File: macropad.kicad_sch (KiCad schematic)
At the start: 6 parts, among them J1 OLED_128x32, SW1 SW_Push, SW2 SW_Push, SW3 SW_Push, SW4 RotaryEncoder_Switch, U1 MOUDLE-SEEEDUINO-XIAO

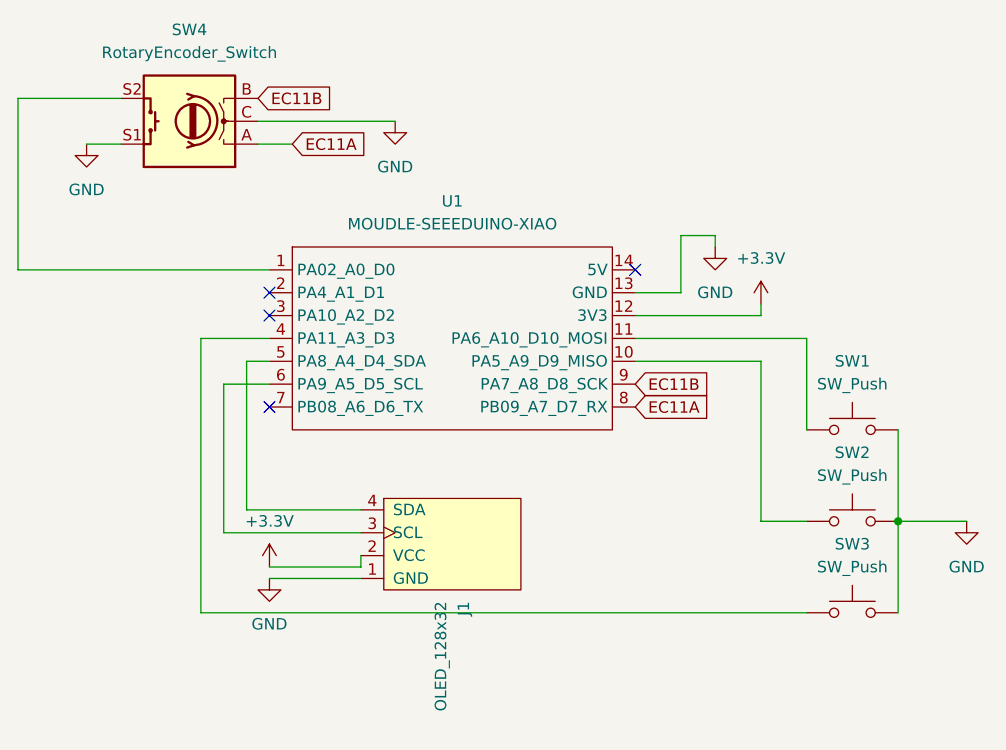
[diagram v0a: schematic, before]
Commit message: changing to simple 3 keys wip
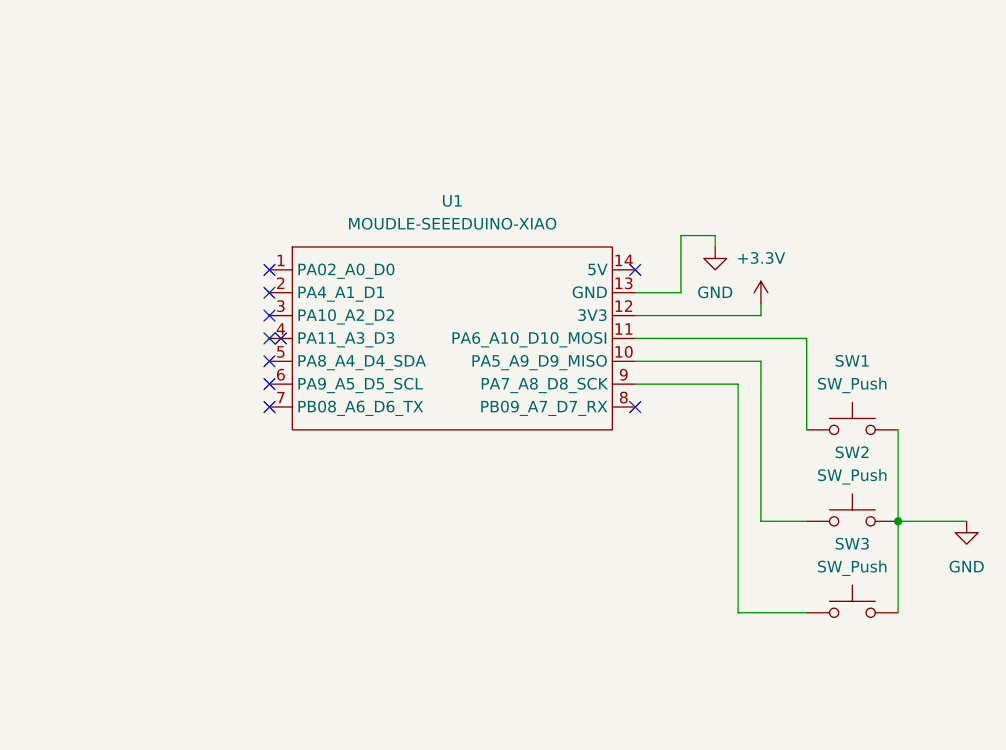
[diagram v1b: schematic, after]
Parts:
- removed J1: OLED_128x32, XIAO_PCB:OLED_128x32, symbol ScottoKeebs:OLED_128x32
- removed SW4: RotaryEncoder_Switch, Rotary_Encoder:RotaryEncoder_Alps_EC11E-Switch_Vertical_H20mm, symbol Device:RotaryEncoder_Switch
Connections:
- net at U1.4 (PA11_A3_D3): no longer SW3.1
- net EC11A: no longer names the net of U1.8 (PB09_A7_D7_RX)
- net EC11B: no longer names the net of U1.9 (PA7_A8_D8_SCK)
- net EC11B: now also SW3.1
- no-connect marks 4 -> 10
